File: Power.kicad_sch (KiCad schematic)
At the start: 26 parts, among them U3 TPS62A02APDDC, U4 TLV75733PDBV, U5 TPS2116DRL

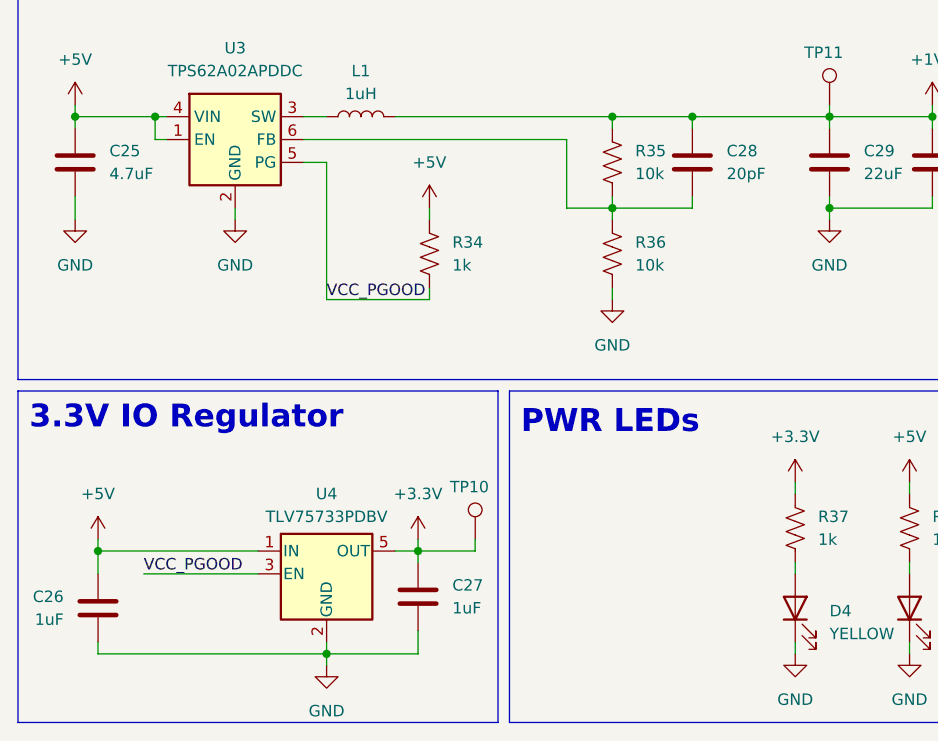
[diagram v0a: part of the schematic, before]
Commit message: Started module-level layout
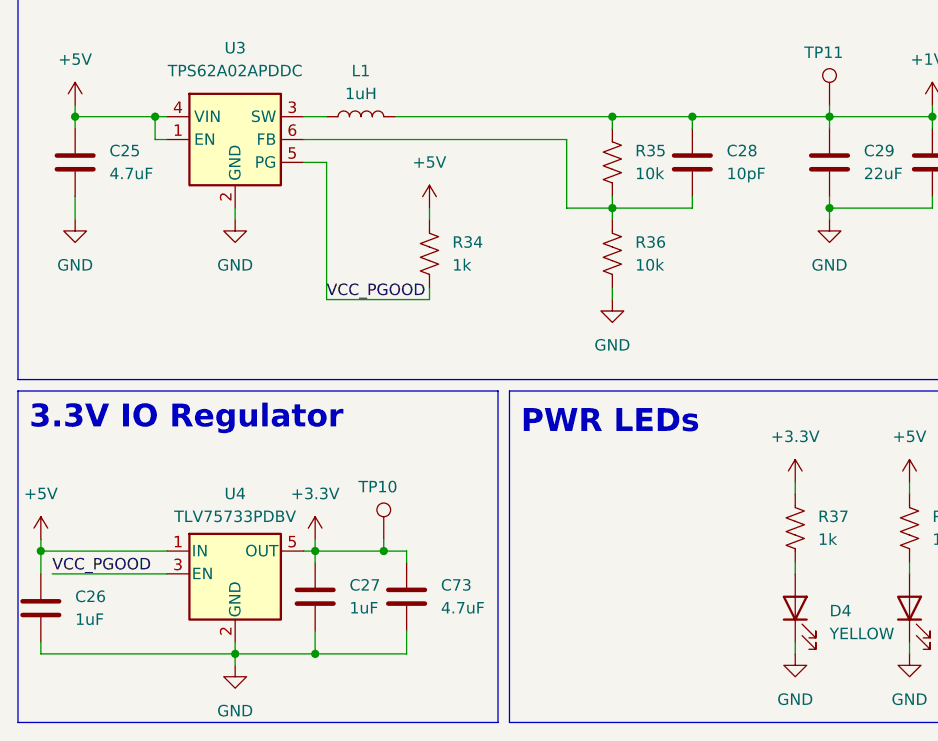
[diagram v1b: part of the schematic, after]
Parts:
- added C73: 4.7uF, Capacitor_SMD:C_0603_1608Metric, symbol Device:C
- C28: value 20pF -> 10pF; Digikey PN 1276-1187-1-ND -> 1276-2149-1-ND
- TP10, TP11, TP12, TP13: footprint TestPoint:TestPoint_Pad_D2.0mm -> TestPoint:TestPoint_Pad_D1.0mm
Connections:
- net +3.3V: now also C73.1
- net GND: now also C73.2
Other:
- moved on the sheet: C26, C27, TP10, U4

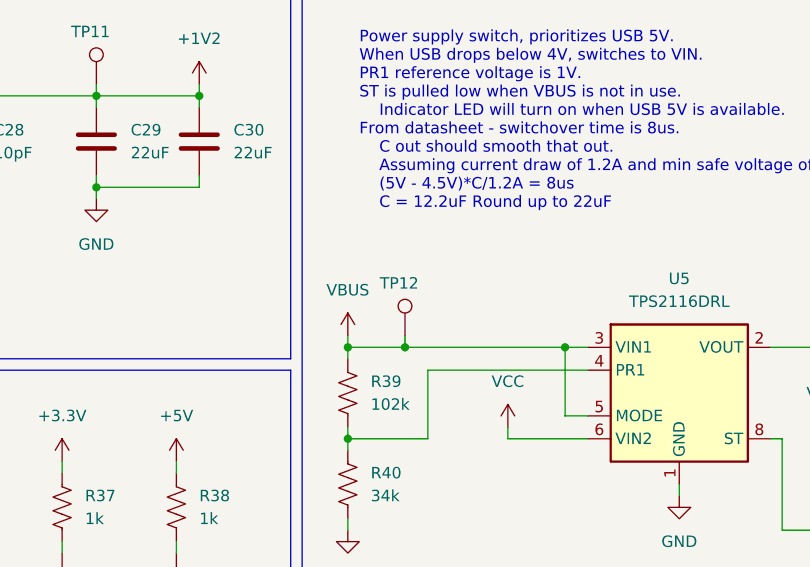
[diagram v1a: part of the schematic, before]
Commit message: Routing done
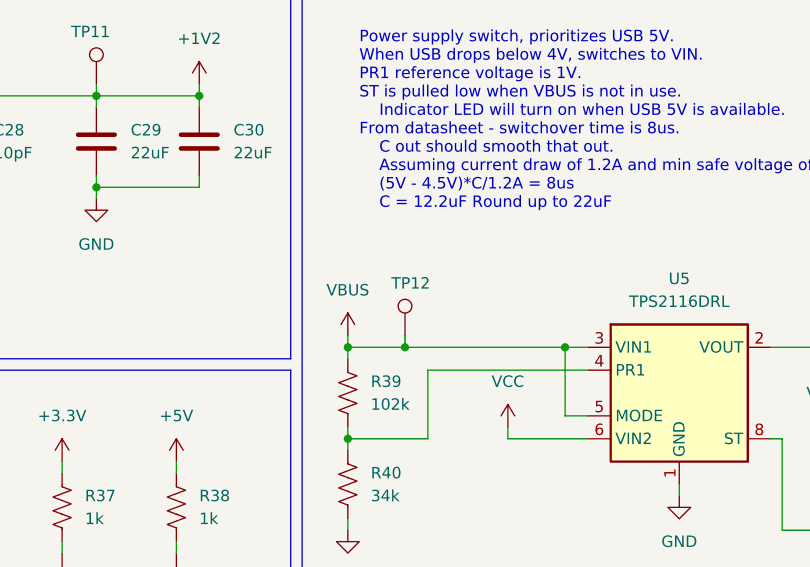
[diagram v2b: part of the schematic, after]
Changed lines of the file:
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@@
 		(lib_id "Connector:TestPoint")
 		(at 163.83 96.52 0)
+		(mirror y)
 		(unit 1)
 		(body_style 1)
@@
 		(dnp no)
 		(property "Reference" "TP12"
-			(at 165.354 90.678 0)
+			(at 162.306 90.678 0)
 			(show_name no)
 			(do_not_autoplace no)
@@
 		)
 		(property "Value" "TestPoint"
-			(at 161.29 91.9481 0)
+			(at 166.37 91.9481 0)
 			(hide yes)
 			(show_name no)
@@
 		)
 		(property "Footprint" "TestPoint:TestPoint_Pad_D1.0mm"
-			(at 168.91 96.52 0)
+			(at 158.75 96.52 0)
 			(hide yes)
 			(show_name no)
@@
 		)
 		(property "Datasheet" ""
-			(at 168.91 96.52 0)
+			(at 158.75 96.52 0)
 			(hide yes)
 			(show_name no)
